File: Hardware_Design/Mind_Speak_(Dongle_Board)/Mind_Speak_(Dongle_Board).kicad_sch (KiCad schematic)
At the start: 26 parts, among them J1 USB_A, J3 Conn_01x05_Pin, J4 Conn_01x05_Pin, SW3 SW_MEC_5E, U1 FT231XQ, U2 NINA-B30x

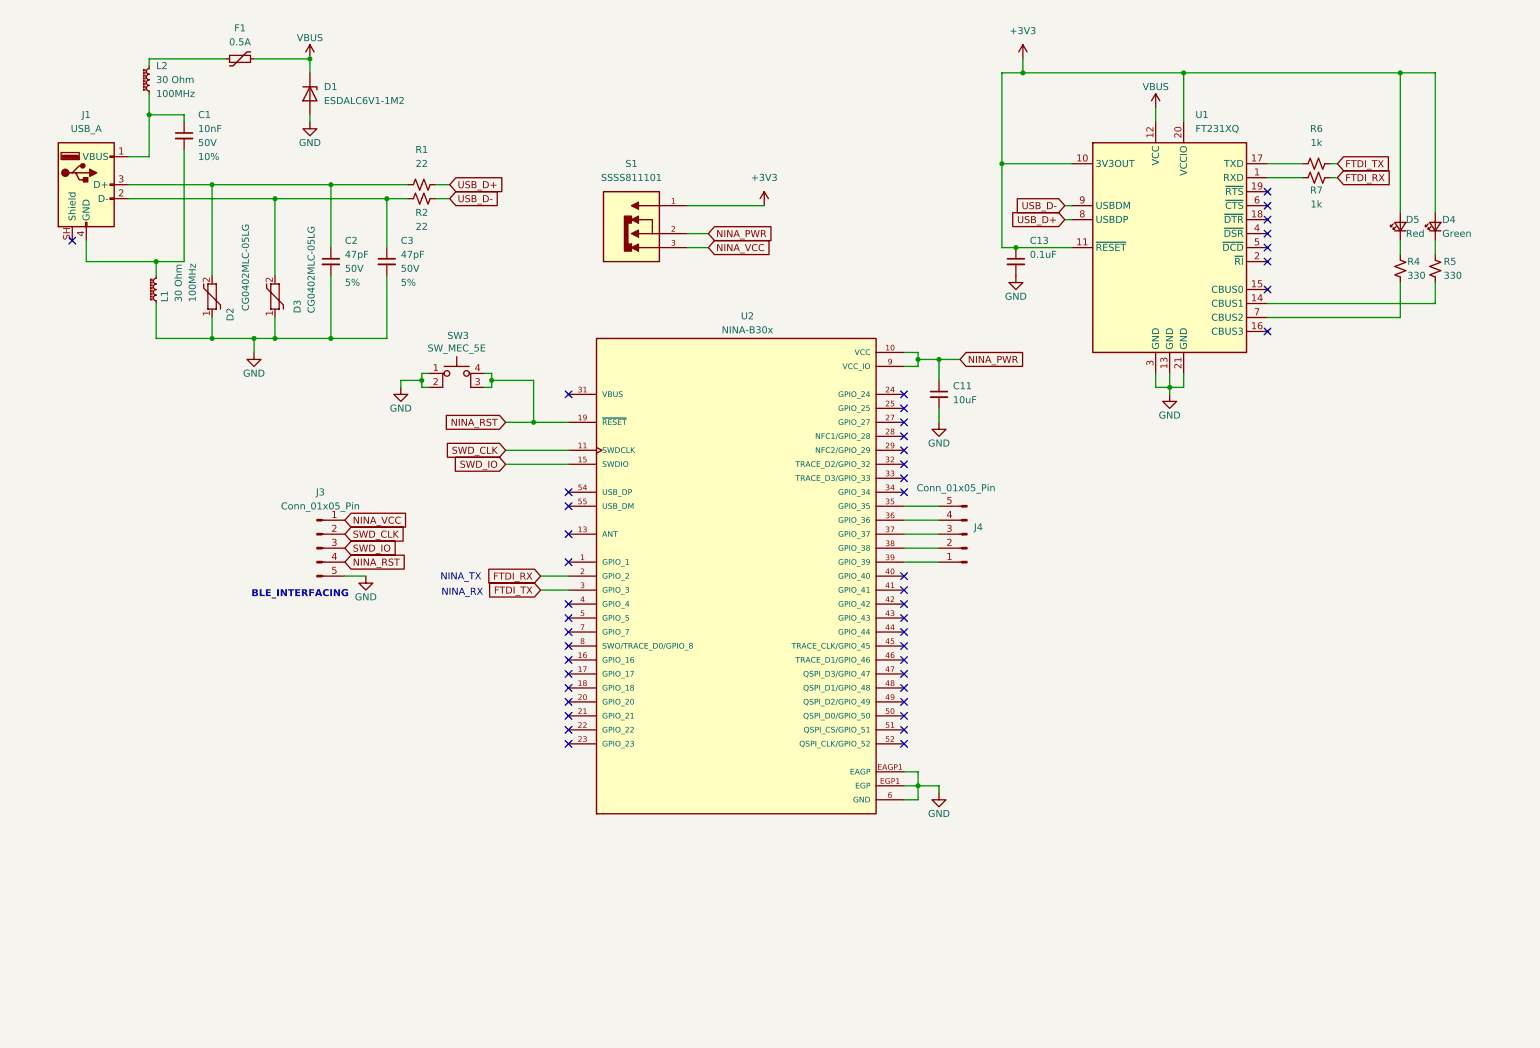
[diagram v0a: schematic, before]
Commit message: Dongle Layout Finished
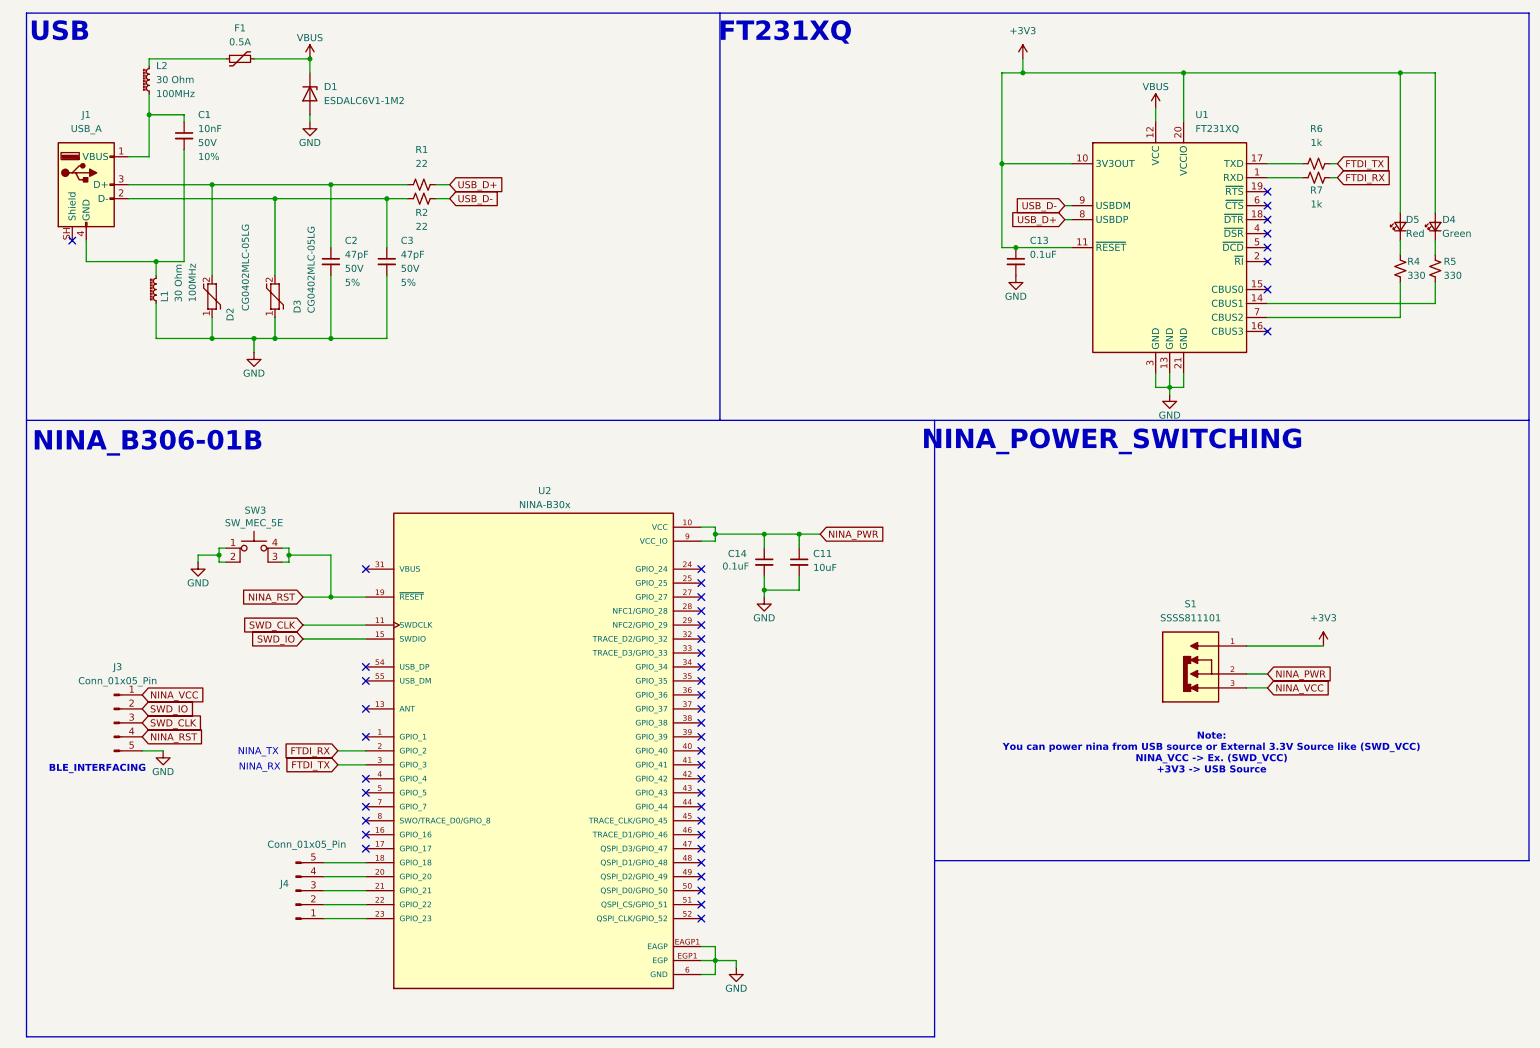
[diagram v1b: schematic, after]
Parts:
- added C14: 0.1uF, PCM_SparkFun-Capacitor:C_0402_1005Metric, symbol PCM_SparkFun-Capacitor:0.1uF_0402_16V_10%
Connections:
- net EAGP: now also C14.2
- net NINA_PWR: now also C14.1
- net SWD_CLK: now also J3.3 (Pin_3); no longer J3.2 (Pin_2)
- net SWD_IO: now also J3.2 (Pin_2); no longer J3.3 (Pin_3)
- net at J4.1 (Pin_1): now also U2.23 (GPIO_23); no longer U2.39 (GPIO_39)
- net at J4.2 (Pin_2): now also U2.22 (GPIO_22); no longer U2.38 (GPIO_38)
- net at J4.3 (Pin_3): now also U2.21 (GPIO_21); no longer U2.37 (GPIO_37)
- net at J4.4 (Pin_4): now also U2.20 (GPIO_20); no longer U2.36 (GPIO_36)
- net at J4.5 (Pin_5): now also U2.18 (GPIO_18); no longer U2.35 (GPIO_35)
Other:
- note added: "FT231XQ"
- note added: "NINA_B306-01B"
- note added: "NINA_POWER_SWITCHING"
- note added: "Note: You can power nina from USB source or External 3.3V Source like (SWD_VCC) NINA_VCC -> Ex. (SWD_VCC) +3V3 -> USB Source"
- note added: "USB"
- moved on the sheet: C11, J3, J4, S1, SW3, U2
